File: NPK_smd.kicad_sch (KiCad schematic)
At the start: 58 parts, among them J2 Screw_Terminal_01x04, J3 USB_C_Receptacle_USB2.0_16P, Q3 SS8050, Q4 SS8050, SW1 SW_Push, SW2 SW_Push, SW3 SW_SPST, U1 AMS1117-3.3, U2 MAX485ESA_T, U3 LM2596S-ADJ, U4 ESP32-WROOM-32, U6 USBLC6-2SC6, U7 CH340C

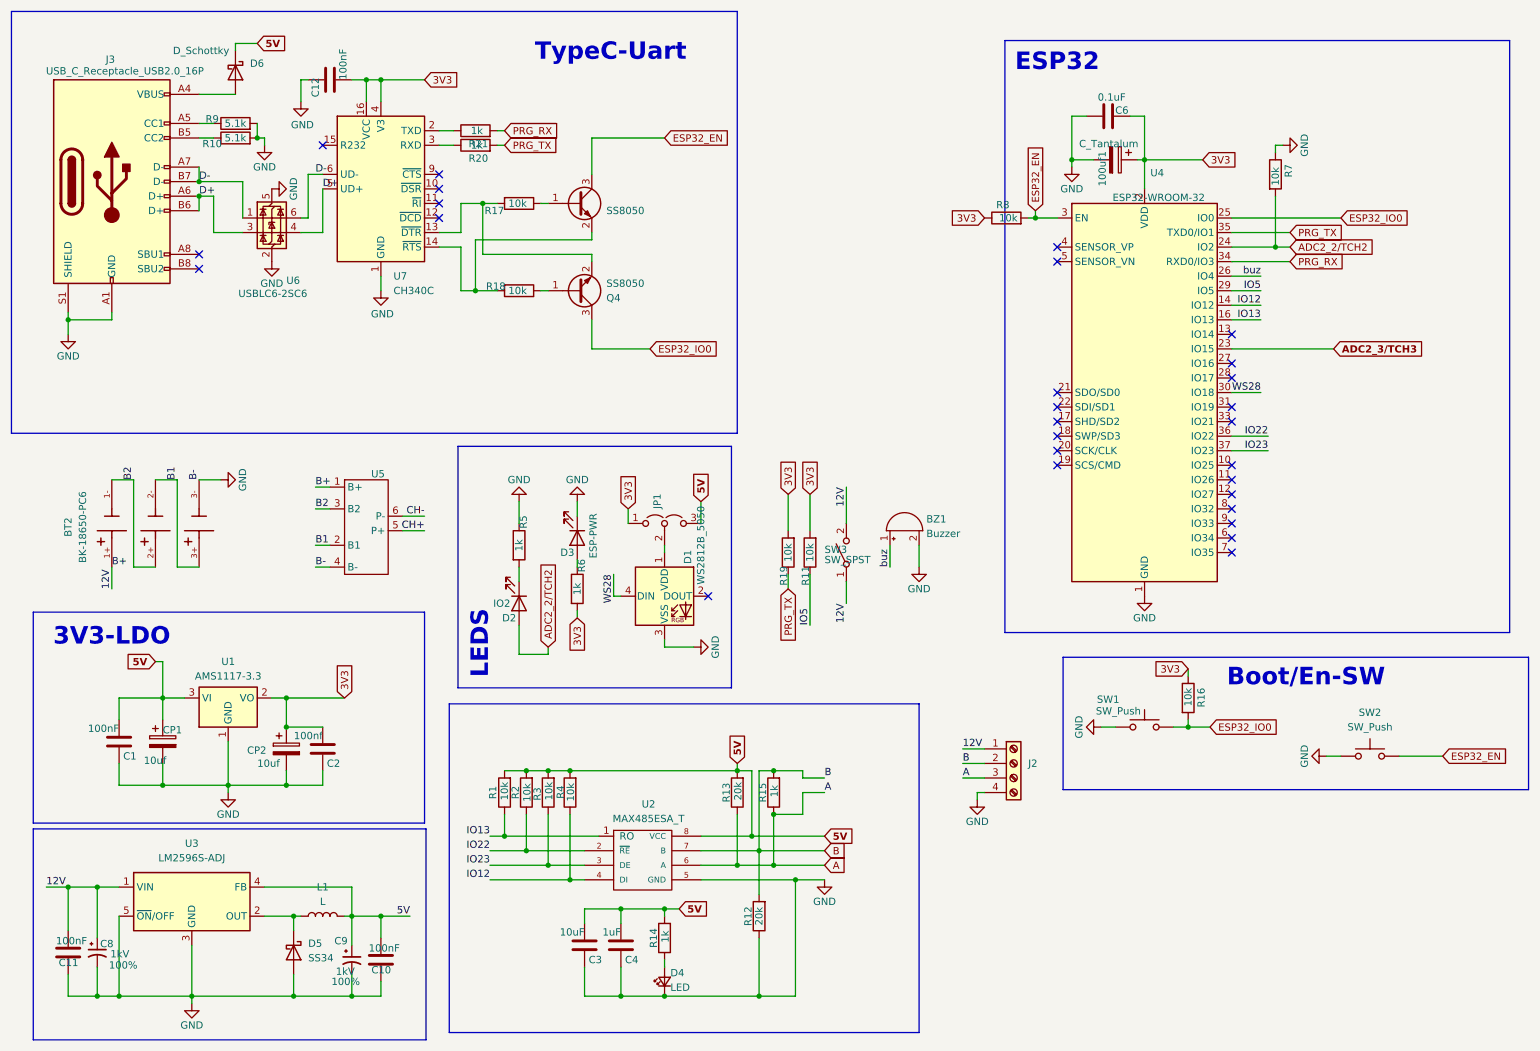
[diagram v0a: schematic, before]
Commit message: updated
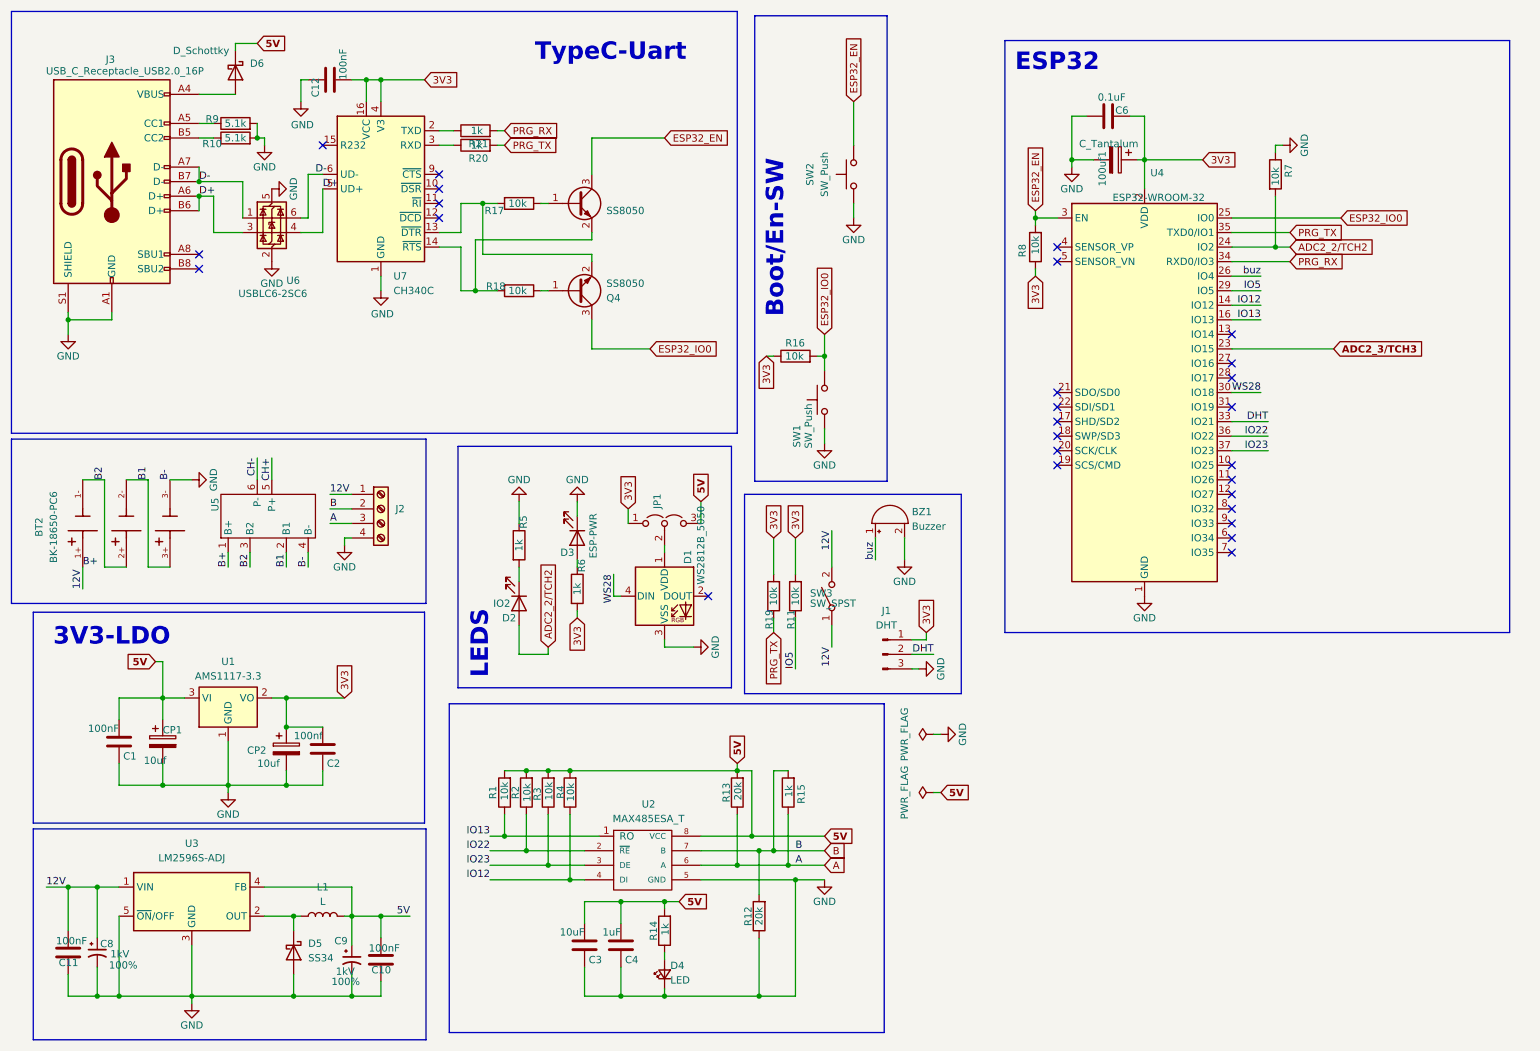
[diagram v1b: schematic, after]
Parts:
- added J1: DHT, Connector_PinSocket_2.54mm:PinSocket_1x03_P2.54mm_Vertical, symbol Connector:Conn_01x03_Pin
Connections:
- net 3V3: now also J1.1 (Pin_1)
- net GND: now also J1.3 (Pin_3)
- net DHT: now reaches U4.33 (IO21)
- net DHT: now also J1.2 (Pin_2)
- no-connect marks 28 -> 27
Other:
- moved on the sheet: BT2, BZ1, D4, J2, R11, R14, R15, R16, R19, R8, SW1, SW2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
